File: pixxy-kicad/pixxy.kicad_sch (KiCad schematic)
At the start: 24 parts, among them Q1 2N3904, SW17 SW_SPDT, U1 Pico

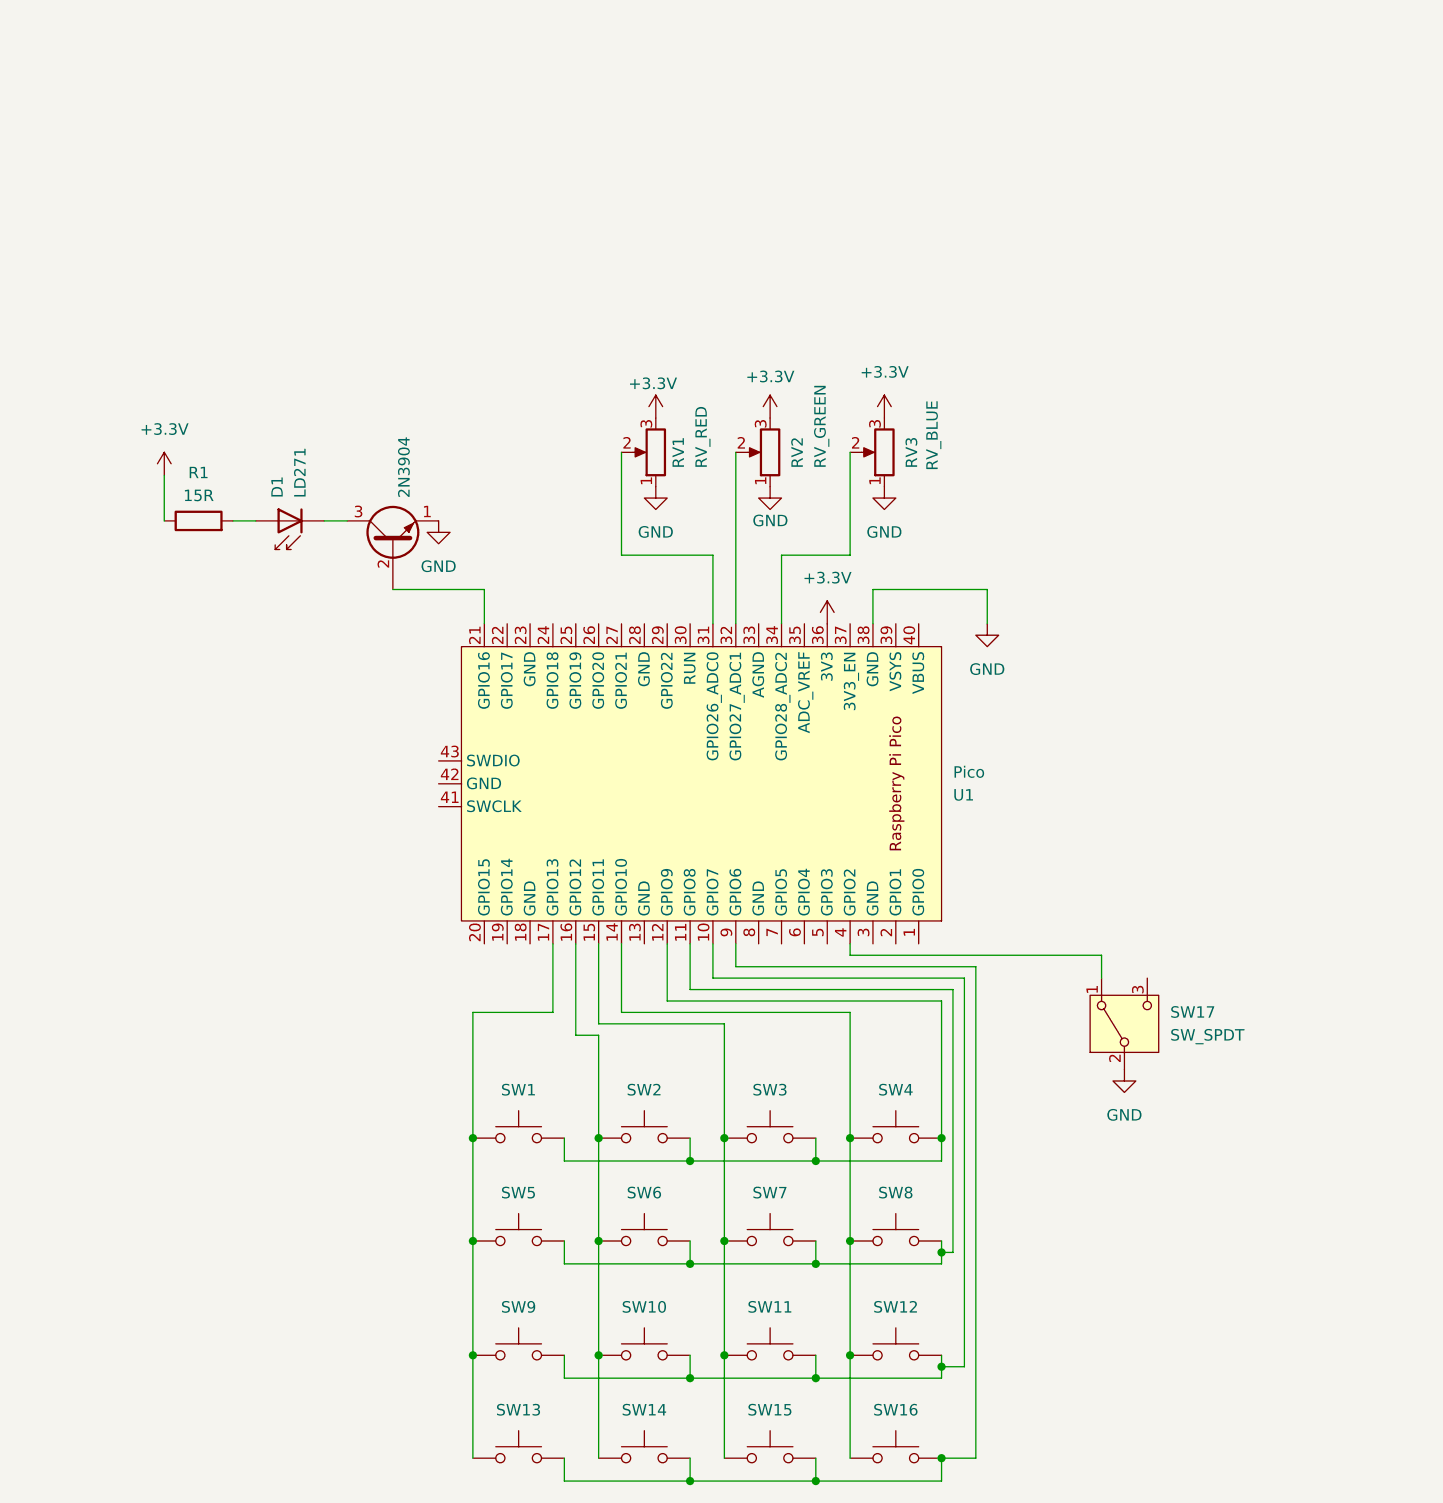
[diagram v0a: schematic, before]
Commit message: Add rev1 pcb files
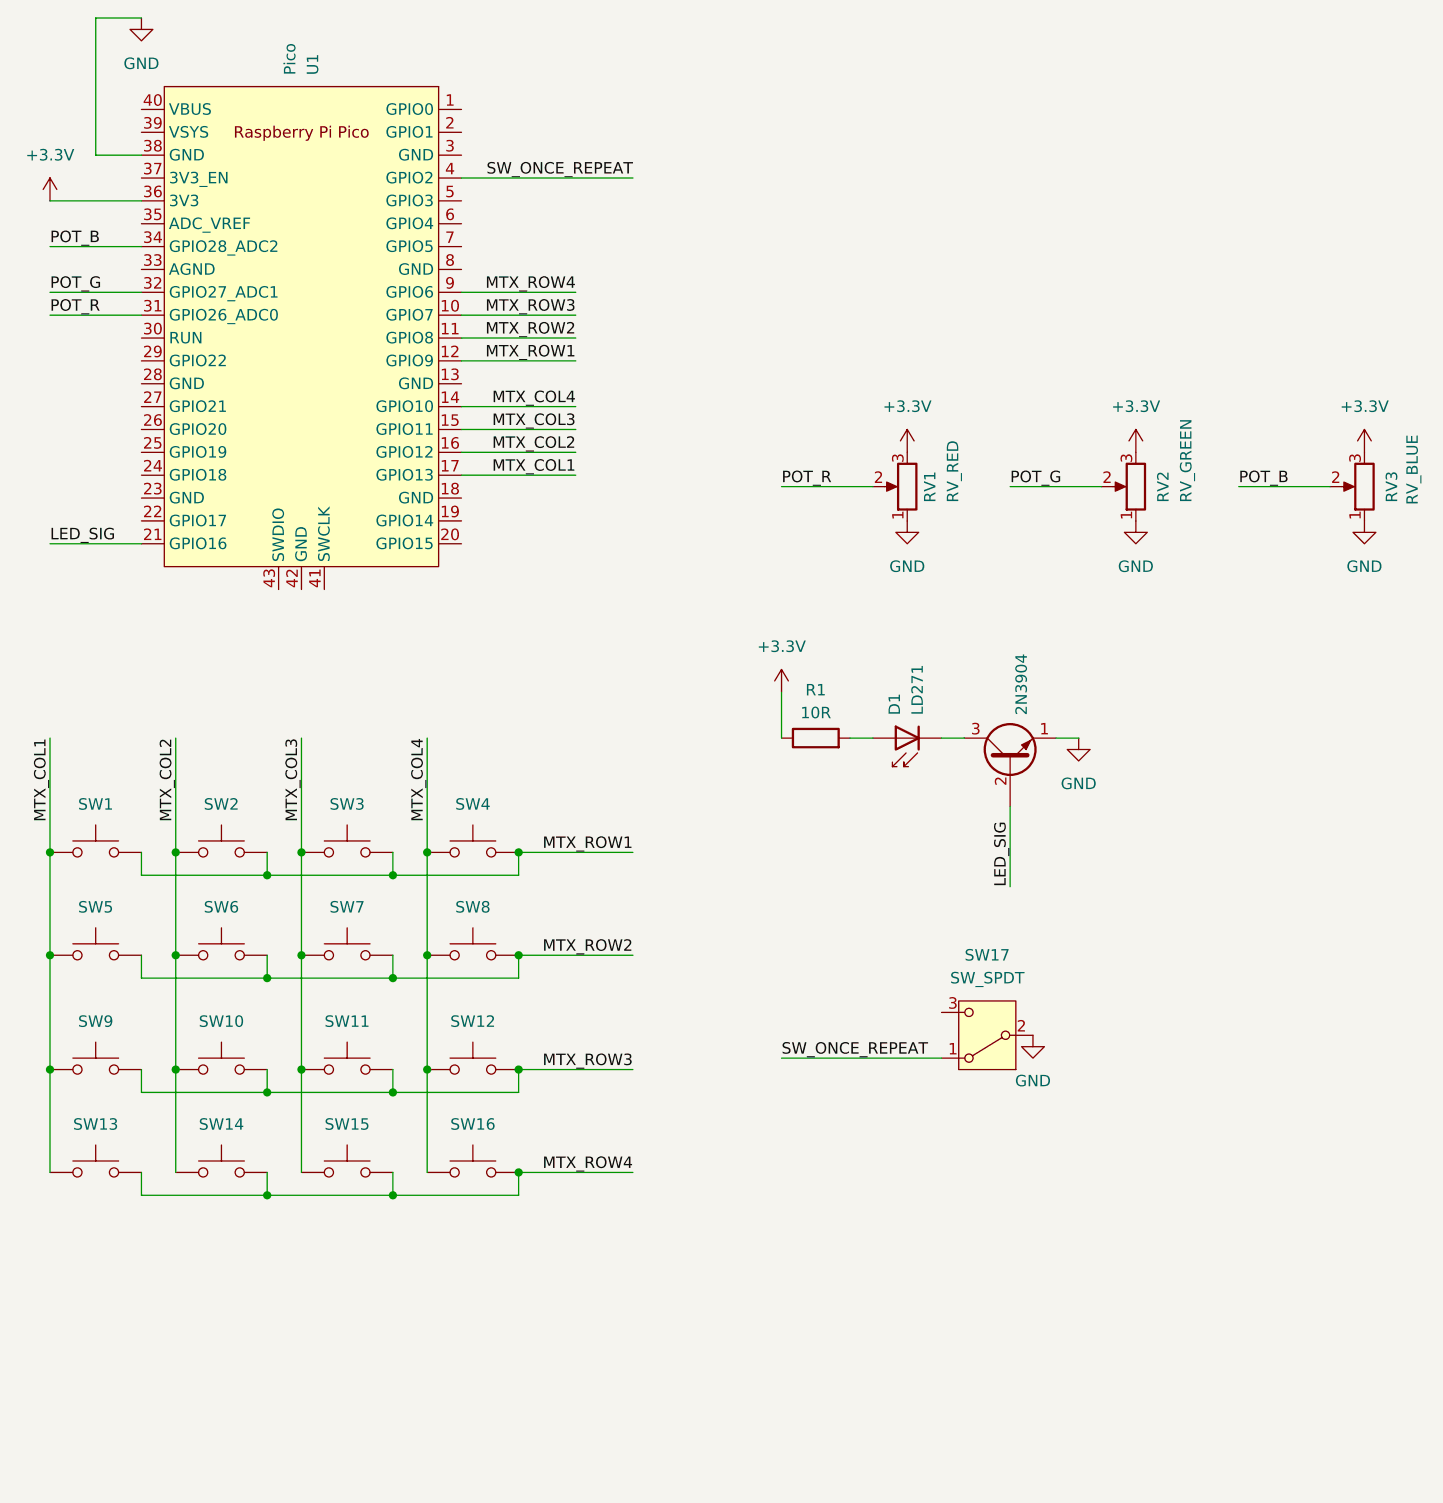
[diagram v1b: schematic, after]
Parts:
- R1: value 15R -> 10R
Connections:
- net MTX_COL2: now reaches SW10.1, SW14.1, SW2.1, SW6.1, U1.16 (GPIO12)
- net MTX_ROW1: now reaches SW1.2, SW2.2, SW3.2, SW4.2, U1.12 (GPIO9)
- net MTX_COL3: now reaches SW11.1, SW15.1, SW3.1, SW7.1, U1.15 (GPIO11)
- net MTX_ROW3: now reaches SW10.2, SW11.2, SW12.2, SW9.2, U1.10 (GPIO7)
- net MTX_COL1: now reaches SW1.1, SW13.1, SW5.1, SW9.1, U1.17 (GPIO13)
- net MTX_ROW2: now reaches SW5.2, SW6.2, SW7.2, SW8.2, U1.11 (GPIO8)
- net MTX_COL4: now reaches SW12.1, SW16.1, SW4.1, SW8.1, U1.14 (GPIO10)
- net POT_G: now reaches RV2.2, U1.32 (GPIO27_ADC1)
- net MTX_ROW4: now reaches SW13.2, SW14.2, SW15.2, SW16.2, U1.9 (GPIO6)
- net POT_B: now reaches RV3.2, U1.34 (GPIO28_ADC2)
- net SW_ONCE_REPEAT: now reaches SW17.1 (A), U1.4 (GPIO2)
- net LED_SIG: now reaches Q1.2 (B), U1.21 (GPIO16)
- net POT_R: now reaches RV1.2, U1.31 (GPIO26_ADC0)
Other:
- moved on the sheet: D1, R1, RV1, RV2, RV3, SW1, SW10, SW11, SW12, SW13, SW14, SW15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
